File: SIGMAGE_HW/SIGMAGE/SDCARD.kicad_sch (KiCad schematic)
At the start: 4 parts, among them J7 473521001

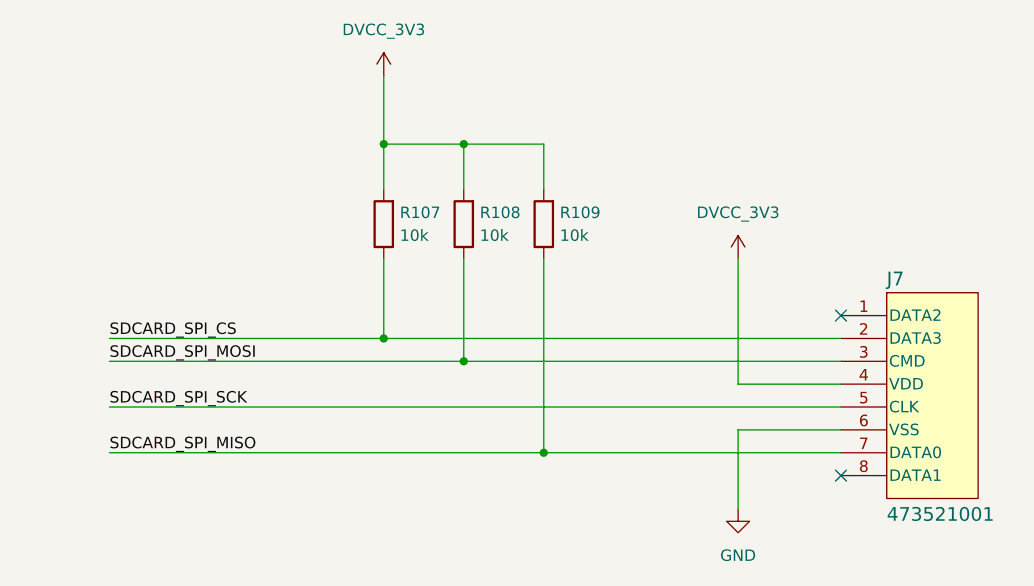
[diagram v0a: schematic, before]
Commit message: changes
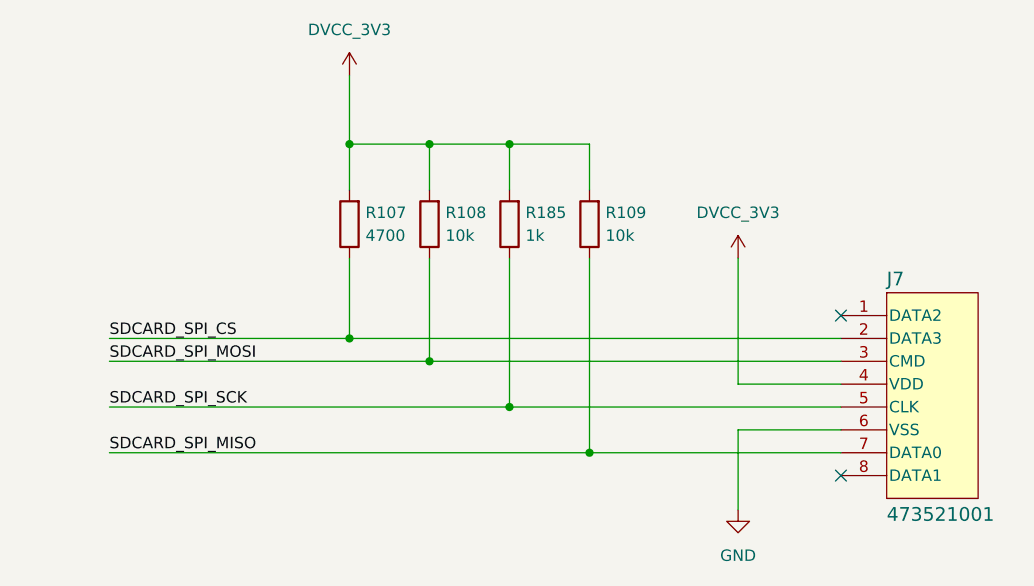
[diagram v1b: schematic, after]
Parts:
- added R185: 1k, Resistor_SMD:R_0603_1608Metric, symbol Device:R
- R107: value 10k -> 4700
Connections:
- net DVCC_3V3: now also R185.2
- net SDCARD_SPI_SCK: now also R185.1
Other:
- moved on the sheet: R107, R108, R109

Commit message: finished schematic
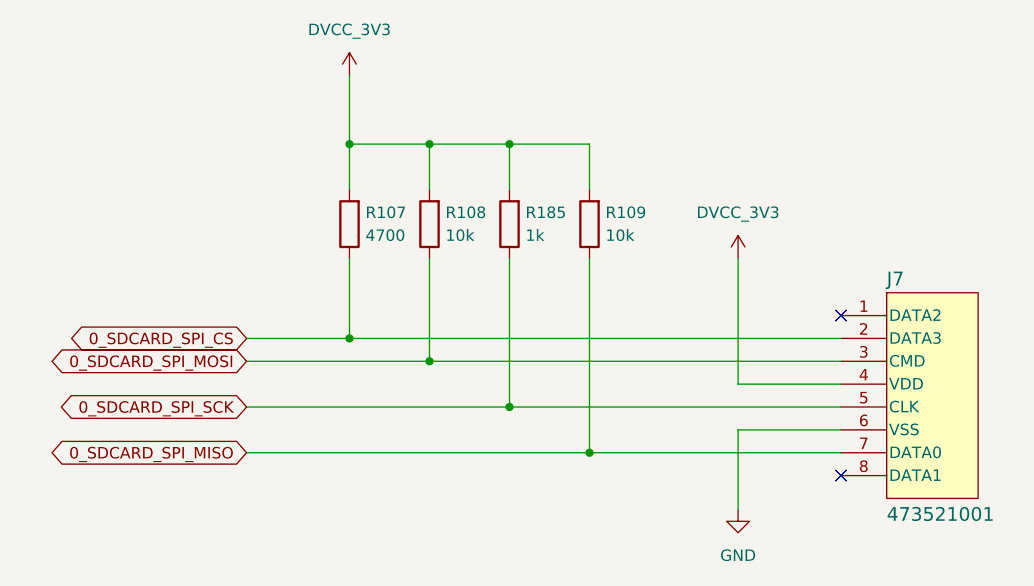
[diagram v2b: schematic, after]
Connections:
- net SDCARD_SPI_CS renamed 0_SDCARD_SPI_CS
- net SDCARD_SPI_MISO renamed 0_SDCARD_SPI_MISO
- net SDCARD_SPI_MOSI renamed 0_SDCARD_SPI_MOSI
- net SDCARD_SPI_SCK renamed 0_SDCARD_SPI_SCK
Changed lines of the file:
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@@
 	(wire
 		(pts
-			(xy 44.45 78.74) (xy 71.12 78.74)
-		)
-		(stroke
-			(width 0)
-			(type default)
-		)
-	)
-	(wire
-		(pts
-			(xy 44.45 86.36) (xy 88.9 86.36)
+			(xy 59.69 78.74) (xy 71.12 78.74)
+		)
+		(stroke
+			(width 0)
+			(type default)
+		)
+	)
+	(wire
+		(pts
+			(xy 59.69 86.36) (xy 88.9 86.36)
 		)
 		(stroke
@@
 	(wire
 		(pts
-			(xy 44.45 81.28) (xy 80.01 81.28)
+			(xy 59.69 81.28) (xy 80.01 81.28)
 		)
 		(stroke
@@
 	(wire
 		(pts
-			(xy 44.45 91.44) (xy 97.79 91.44)
+			(xy 59.69 91.44) (xy 97.79 91.44)
 		)
 		(stroke
@@
 		)
 	)
-	(label "SDCARD_SPI_MOSI"
-		(at 44.45 81.28 0)
-		(effects
-			(font
-				(size 1.27 1.27)
-			)
-			(justify left bottom)
-		)
-	)
-	(label "SDCARD_SPI_SCK"
-		(at 44.45 86.36 0)
-		(effects
-			(font
-				(size 1.27 1.27)
-			)
-			(justify left bottom)
-		)
-	)
-	(label "SDCARD_SPI_MISO"
-		(at 44.45 91.44 0)
-		(effects
-			(font
-				(size 1.27 1.27)
-			)
-			(justify left bottom)
-		)
-	)
-	(label "SDCARD_SPI_CS"
-		(at 44.45 78.74 0)
-		(effects
-			(font
-				(size 1.27 1.27)
-			)
-			(justify left bottom)
-		)
-	)
+	(global_label "0_SDCARD_SPI_CS"
+		(shape bidirectional)
+		(at 59.69 78.74 180)
+		(fields_autoplaced yes)
+		(effects
+			(font
+				(size 1.27 1.27)
+			)
+			(justify right)
+		)
+		(property "Intersheetrefs" "${INTERSHEET_REFS}"
+			(at 38.5393 78.74 0)
+			(hide yes)
+			(show_name no)
+			(do_not_autoplace no)
+			(effects
+				(font
+					(size 1.27 1.27)
+				)
+				(justify right)
+			)
+		)
+	)
+	(global_label "0_SDCARD_SPI_MISO"
+		(shape bidirectional)
+		(at 59.69 91.44 180)
+		(fields_autoplaced yes)
+		(effects
+			(font
+				(size 1.27 1.27)
+			)
+			(justify right)
+		)
+		(property "Intersheetrefs" "${INTERSHEET_REFS}"
+			(at 36.4226 91.44 0)
+			(hide yes)
+			(show_name no)
+			(do_not_autoplace no)
+			(effects
+				(font
+					(size 1.27 1.27)
+				)
+				(justify right)
+			)
+		)
+	)
+	(global_label "0_SDCARD_SPI_MOSI"
+		(shape bidirectional)
+		(at 59.69 81.28 180)
+		(fields_autoplaced yes)
+		(effects
+			(font
+				(size 1.27 1.27)
+			)
+			(justify right)
+		)
+		(property "Intersheetrefs" "${INTERSHEET_REFS}"
+			(at 36.4226 81.28 0)
+			(hide yes)
+			(show_name no)
+			(do_not_autoplace no)
+			(effects
+				(font
+					(size 1.27 1.27)
+				)
+				(justify right)
+			)
+		)
+	)
+	(global_label "0_SDCARD_SPI_SCK"
+		(shape bidirectional)
+		(at 59.69 86.36 180)
+		(fields_autoplaced yes)
+		(effects
+			(font
+				(size 1.27 1.27)
+			)
+			(justify right)
+		)
+		(property "Intersheetrefs" "${INTERSHEET_REFS}"
+			(at 37.2693 86.36 0)
+			(hide yes)
+			(show_name no)
+			(do_not_autoplace no)
+			(effects
+				(font
+					(size 1.27 1.27)
+				)
+				(justify right)
+			)
+		)
+	)
